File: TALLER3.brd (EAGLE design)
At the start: 77.1 x 49.5 mm, 11 parts, among them IC1 LM741P, J2 1X5, K1 JJM1-12V, T1 2N3904

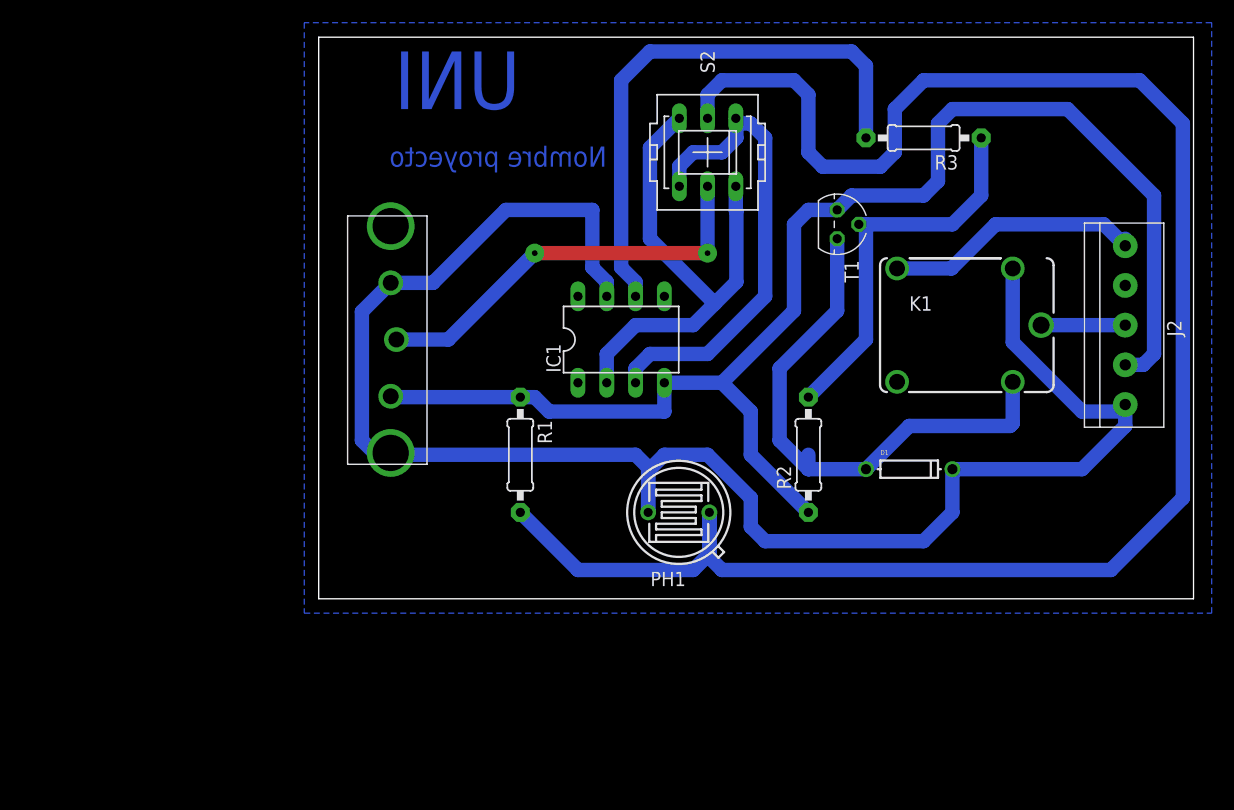
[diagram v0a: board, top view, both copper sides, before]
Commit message: RAS UNI 08/06/2019.
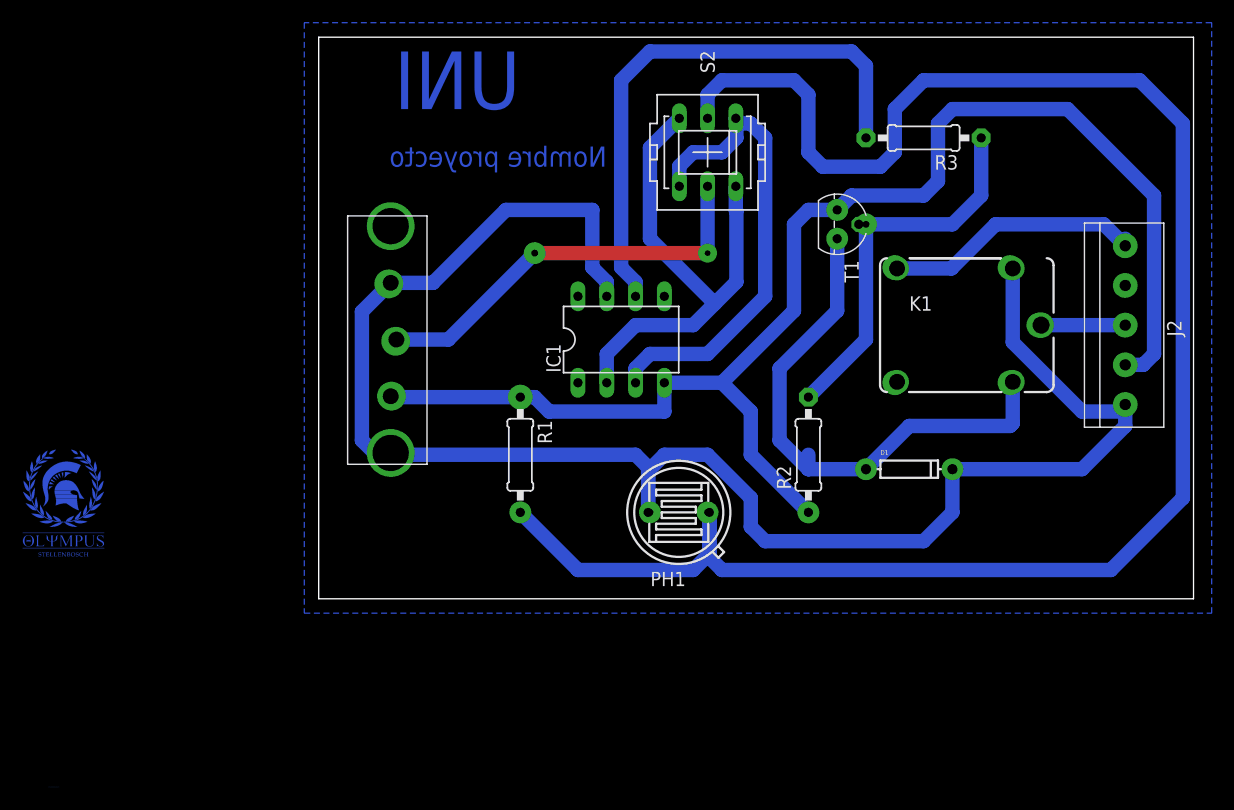
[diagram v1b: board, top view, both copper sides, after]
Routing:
- net V+: vias 0 -> 1
- net N$9: vias 0 -> 2
- net N$8: vias 0 -> 1
- net GNDA: vias 0 -> 3
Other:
- board text added: "C:/Users/yesse/Desktop/olympus2.bmp"
